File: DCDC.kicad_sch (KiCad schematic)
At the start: 34 parts, among them U3 TPS63021DSJR, U4 TPS61088RHLR

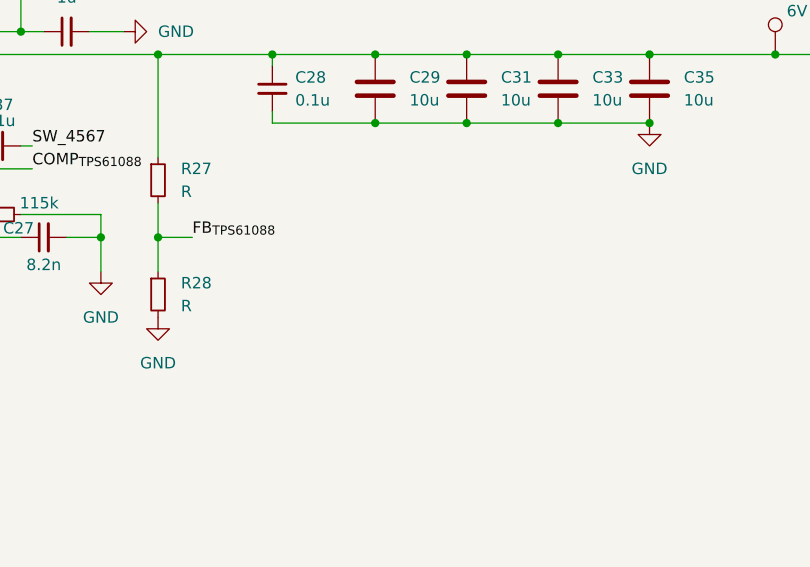
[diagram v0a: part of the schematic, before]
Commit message: update
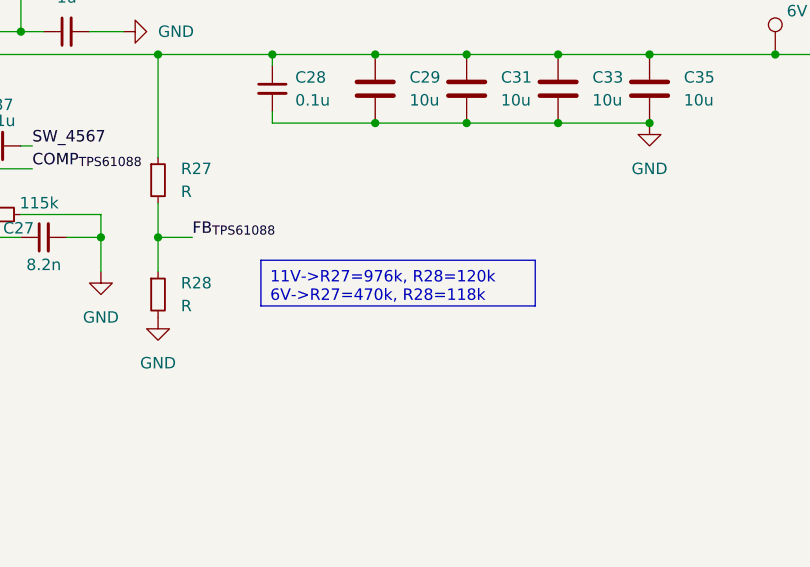
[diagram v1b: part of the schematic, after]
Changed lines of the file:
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@@
+		)
+	)
+	(text_box "11V->R27=976k, R28=120k\n6V->R27=470k, R28=118k\n"
+		(exclude_from_sim no)
+		(at 194.31 134.62 0)
+		(size 30.48 5.08)
+		(stroke
+			(width 0)
+			(type default)
+		)
+		(fill
+			(type none)
+		)
+		(effects
+			(font
+				(size 1.27 1.27)
+			)
+			(justify left top)
 		)
 	)
